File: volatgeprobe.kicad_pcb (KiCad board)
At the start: 2 copper layers, 107 x 49 mm, 52 parts, among them IC1 AMC1301SDWV, J1 Conn_01x01_Male, J2 Conn_01x01_Male, J3 Conn_01x02_Male, J4 Conn_Coaxial, SW1 SW_SPST, U1 AZ1117IH-3.3TRG1, U2 5-15v, U4 LF353M, U5 LF353M

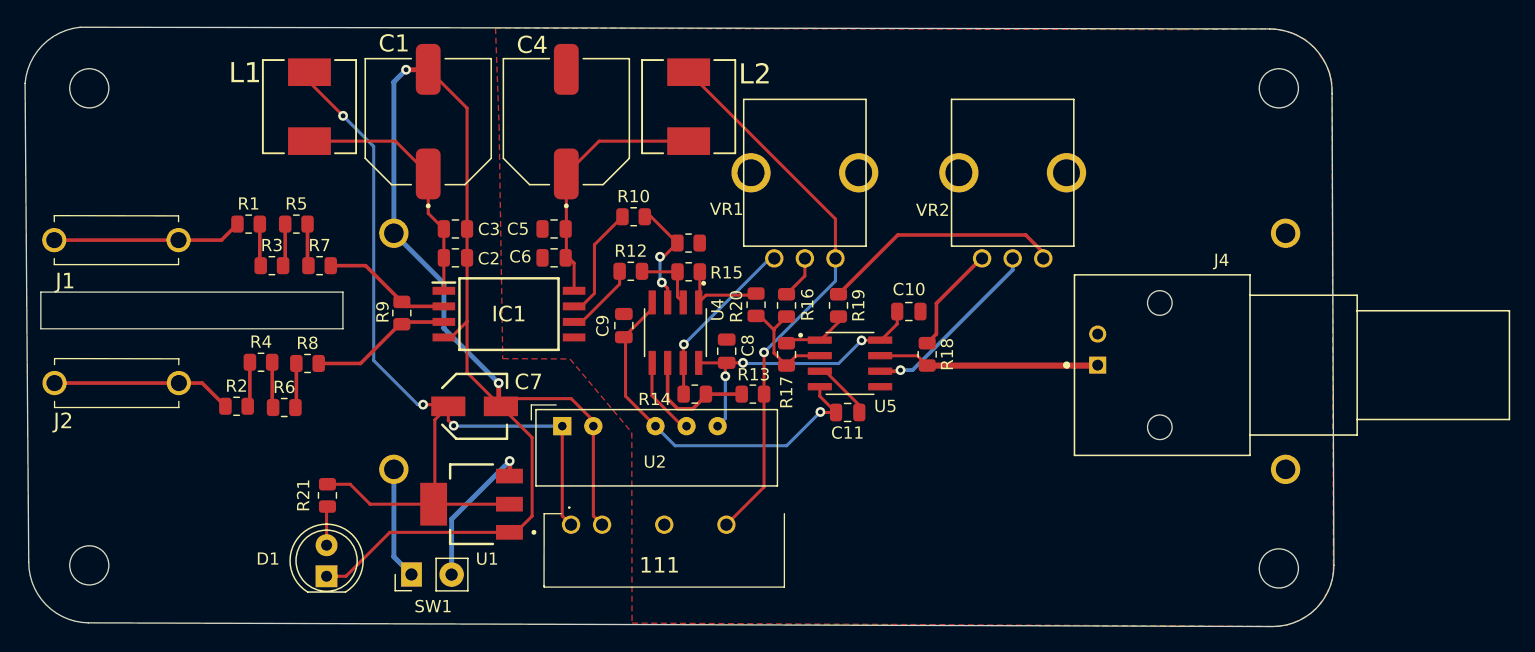
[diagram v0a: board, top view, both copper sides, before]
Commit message: changed
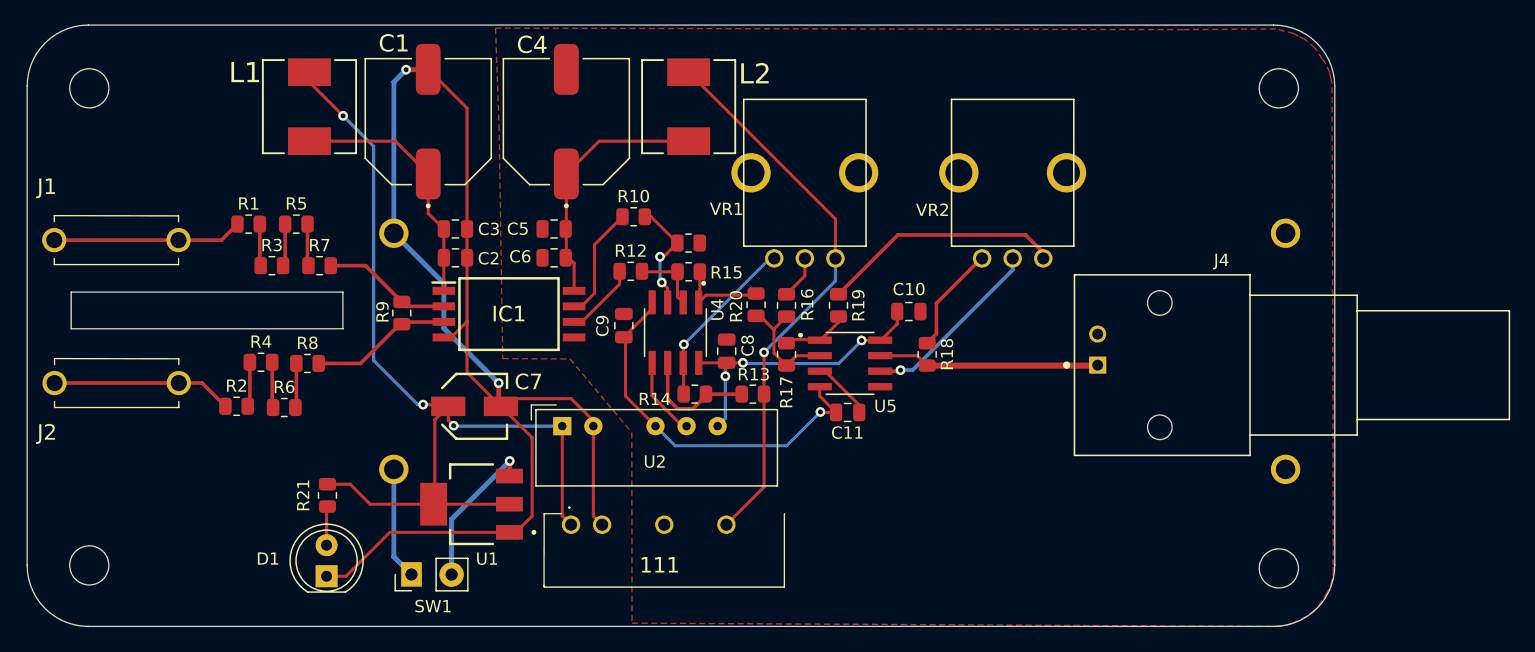
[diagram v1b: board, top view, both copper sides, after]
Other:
- board size 107 x 49 mm -> 106.9 x 49.2 mm
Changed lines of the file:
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@@
     (property "ki_keywords" "connector")
     (attr through_hole)
-    (fp_text reference "J2" (at 0.72 3.105 180) (layer "F.SilkS")
+    (fp_text reference "J2" (at -0.61 4.045 180) (layer "F.SilkS")
         (effects (font (size 1.27 1.27) (thickness 0.254)))
     )
@@
     (property "ki_keywords" "connector")
     (attr through_hole)
-    (fp_text reference "J1" (at 0.9025 3.35) (layer "F.SilkS")
+    (fp_text reference "J1" (at -0.5875 -4.36) (layer "F.SilkS")
         (effects (font (size 1.27 1.27) (thickness 0.254)))
     )
@@
       (solder_mask_margin 0.1016))
   )
-  (gr_arc (start 96.76625 84.71) (mid 98.184413 81.598526) (end 101.267142 80.118919)
+  (gr_arc (start 101.93625 129.1) (mid 98.400716 127.635534) (end 96.93625 124.1)
     (stroke (width 0.1) (type default)) (layer "Edge.Cuts"))
-  (gr_line (start 101.267142 80.118919) (end 198.51625 80.25608)
+  (gr_arc (start 96.93625 84.94) (mid 98.400719 81.404484) (end 101.93625 79.94)
     (stroke (width 0.1) (type default)) (layer "Edge.Cuts"))
-  (gr_rect (start 98.05625 101.77) (end 122.75625 104.77)
+  (gr_line (start 198.83625 129.1) (end 101.93625 129.1)
+    (stroke (width 0.1) (type default)) (layer "Edge.Cuts"))
+  (gr_line (start 101.93625 79.94) (end 198.83625 79.94)
+    (stroke (width 0.1) (type default)) (layer "Edge.Cuts"))
+  (gr_arc (start 203.83625 124.1) (mid 202.371784 127.635534) (end 198.83625 129.1)
+    (stroke (width 0.1) (type default)) (layer "Edge.Cuts"))
+  (gr_rect (start 100.53625 101.77) (end 122.75625 104.77)
     (stroke (width 0.1) (type default)) (fill none) (layer "Edge.Cuts"))
-  (gr_arc (start 198.51625 80.25608) (mid 202.195298 81.822401) (end 203.61625 85.56)
+  (gr_arc (start 198.83625 79.94) (mid 202.371784 81.404466) (end 203.83625 84.94)
     (stroke (width 0.1) (type default)) (layer "Edge.Cuts"))
-  (gr_line (start 97.065682 123.86) (end 96.76625 84.71)
+  (gr_line (start 203.83625 84.94) (end 203.83625 124.1)
     (stroke (width 0.1) (type default)) (layer "Edge.Cuts"))
-  (gr_arc (start 101.94125 128.81) (mid 98.489253 127.333963) (end 97.065682 123.86)
-    (stroke (width 0.1) (type default)) (layer "Edge.Cuts"))
-  (gr_line (start 198.76625 129.11) (end 101.94125 128.81)
-    (stroke (width 0.1) (type default)) (layer "Edge.Cuts"))
-  (gr_arc (start 203.76625 124.11) (mid 202.301784 127.645534) (end 198.76625 129.11)
-    (stroke (width 0.1) (type default)) (layer "Edge.Cuts"))
-  (gr_line (start 203.61625 85.56) (end 203.76625 124.11)
+  (gr_line (start 96.93625 124.1) (end 96.93625 84.94)
     (stroke (width 0.1) (type default)) (layer "Edge.Cuts"))
   (gr_text "check banana jack size" (at 154.94625 70.07) (layer "Cmts.User")
